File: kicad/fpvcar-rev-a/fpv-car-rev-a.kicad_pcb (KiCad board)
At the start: 2 copper layers, 58 parts, among them J1 CAMERA, J10 GPIO, J11 USB C, J12 GPIO, J13 GPIO, J14 RGB FL, J15 RGB FR, J16 RGB BL, J17 RGB BR, J2 Steering, J4 Battery, J5 Debug UART, J6 M1, J7 M2, J8 NRF24L01, J9 GPIO, Q1 Q_PMOS_GSD, SW1 SW_SPST, SW2 SW_SPST, U1 ESP32-S3-WROOM-1, U2 AMS1117-5.0, U3 XC6206-1.2V, U4 XC6206-2.8V, U5 DRV8833PWP, U6 WL2803K33-5/TR

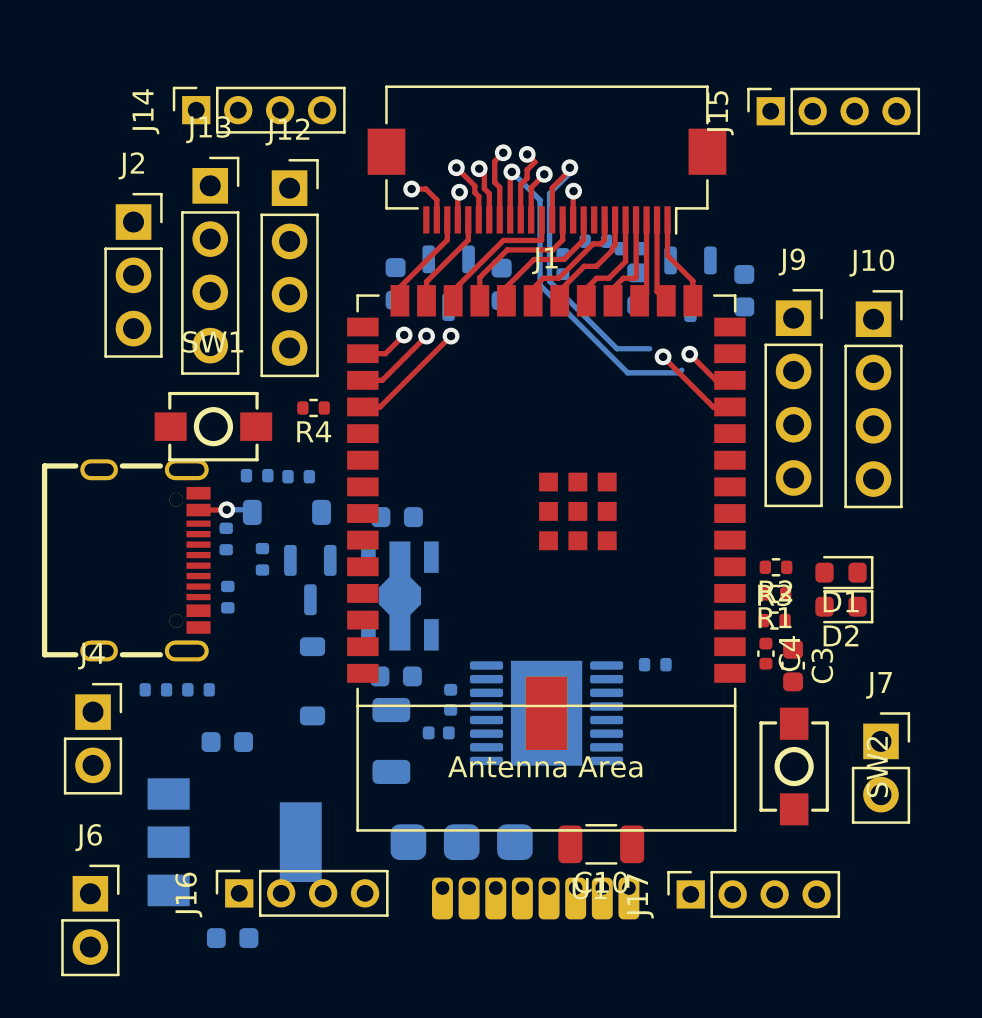
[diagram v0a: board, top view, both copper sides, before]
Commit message: PCB for rev. A done!
PCB name: S3Voyager :)
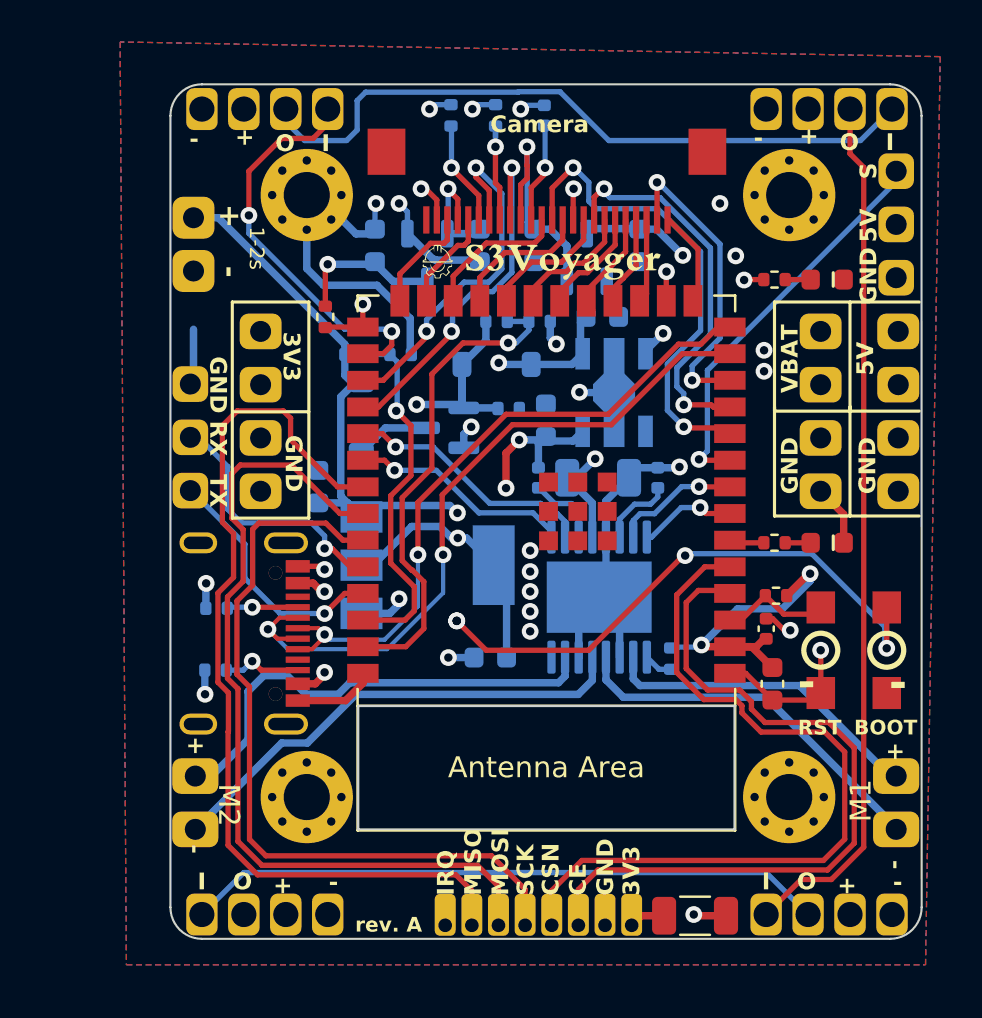
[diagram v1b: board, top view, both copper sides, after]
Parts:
- removed J10, J13: GPIO, Connector_PinSocket_2.54mm:PinSocket_1x04_P2.54mm_Vertical
- added H1: MountingHole_Pad, MountingHole:MountingHole_2.2mm_M2_Pad_Via, F.Cu at (164.0, 96.3)
- added H2: MountingHole_Pad, MountingHole:MountingHole_2.2mm_M2_Pad_Via, F.Cu at (141.0, 96.3)
- added H3: MountingHole_Pad, MountingHole:MountingHole_2.2mm_M2_Pad_Via, F.Cu at (141.0, 125.0)
- added H4: MountingHole_Pad, MountingHole:MountingHole_2.2mm_M2_Pad_Via, F.Cu at (164.0, 125.0)
- added J3: Bat Power, Custom3:conn_01x04, F.Cu at (165.5, 102.8)
- D1: renamed from D2; value BLUE -> RED
- D2: renamed from D1; value RED -> BLUE
- J12: value GPIO -> 3.3V Power; footprint Connector_PinSocket_2.54mm:PinSocket_1x04_P2.54mm_Vertical -> Custom3:conn_01x04
- J14, J15, J16, J17: footprint Connector_PinSocket_2.00mm:PinSocket_1x04_P2.00mm_Vertical -> Custom3:RGB_4_Pin_2mm_Female
- J9: value GPIO -> 5V Power; footprint Connector_PinSocket_2.54mm:PinSocket_1x04_P2.54mm_Vertical -> Custom3:conn_01x04
- moved J2 36.4 mm to (169.1, 95.2)
- moved SW1 33.8 mm to (168.7, 118.0), turned to -90 degrees
- moved J4 24.1 mm to (135.6, 97.4)
- moved J5 19.7 mm to (135.4, 110.4), turned to 0 degrees
- moved R12 18.7 mm to (145.5, 103.9)
- moved R11 18.6 mm to (143.3, 103.9)
- moved C1 18.2 mm to (149.8, 118.3)
- moved U2 16.1 mm to (146.8, 113.9)
- moved C9 16.0 mm to (154.9, 109.8), turned to 0 degrees
- moved C11 14.5 mm to (157.7, 109.8), turned to -90 degrees
- moved C15 14.1 mm to (152.4, 107.0), turned to 90 degrees
- moved U6 14.1 mm to (155.7, 105.7)
- moved D2 14.0 mm to (165.8, 100.3)
- moved R10 13.8 mm to (150.6, 106.5), turned to 0 degrees
- moved R2 13.7 mm to (163.3, 100.3), turned to 0 degrees
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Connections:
- net NRF_IRQ renamed /NRF_IRQ
- D1 pad 2: Net-(D2-A) -> Net-(D1-A)
- D2 pad 2: Net-(D1-A) -> Net-(D2-A)
- J12 pad 1: GPIO00 -> +3.3V
- J12 pad 2: GPIO00 -> +3.3V
- J12 pad 3: +3.3V -> GND
- J16 pad 1: /RGB_FR_BL -> /RGB_BL_BR
- J16 pad 2: /RGB_BL_BR -> unconnected-(J16-Pin_2-Pad2)
- J17 pad 1: /RGB_BL_BR -> /RGB_FR_BL
- J17 pad 2: unconnected-(J17-Pin_2-Pad2) -> /RGB_BL_BR
- J6 pad 1: MOTOR_A_OUT1 -> MOTOR_B_OUT1
- J6 pad 2: MOTOR_A_OUT2 -> MOTOR_B_OUT2
- J7 pad 1: MOTOR_B_OUT1 -> MOTOR_A_OUT1
- J7 pad 2: MOTOR_B_OUT2 -> MOTOR_A_OUT2
- J9 pad 1: GPIO00 -> +5V
- J9 pad 2: GPIO00 -> +5V
- J9 pad 3: +5V -> GND
- U1 pad 10: unconnected-(U1-GPIO17/U1TXD/ADC2_CH6-Pad10) -> XCLK
- U1 pad 11: unconnected-(U1-GPIO18/U1RXD/ADC2_CH7/CLK_OUT3-Pad11) -> PCLK
- U1 pad 12: unconnected-(U1-GPIO8/TOUCH8/ADC1_CH7/SUBSPICS1-Pad12) -> DATA1
- U1 pad 16: DATA1 -> LED_BLUE
- U1 pad 28: unconnected-(U1-SPIIO6/GPIO35/FSPID/SUBSPID-Pad28) -> RGB_LED
- U1 pad 29: unconnected-(U1-SPIIO7/GPIO36/FSPICLK/SUBSPICLK-Pad29) -> VSYNC
- U1 pad 30: unconnected-(U1-SPIDQS/GPIO37/FSPIQ/SUBSPIQ-Pad30) -> HREF
- U1 pad 31: unconnected-(U1-GPIO38/FSPIWP/SUBSPIWP-Pad31) -> MOTOR_B_IN2
- U1 pad 32: unconnected-(U1-MTCK/GPIO39/CLK_OUT3/SUBSPICS1-Pad32) -> MOTOR_B_IN1
- U1 pad 33: unconnected-(U1-MTDO/GPIO40/CLK_OUT2-Pad33) -> NRF_MISO
- U1 pad 34: unconnected-(U1-MTDI/GPIO41/CLK_OUT1-Pad34) -> NRF_MOSI
- U1 pad 35: unconnected-(U1-MTMS/GPIO42-Pad35) -> NRF_SCK
- U1 pad 38: unconnected-(U1-GPIO2/TOUCH2/ADC1_CH1-Pad38) -> BATT_VOLTAGE
- U1 pad 39: unconnected-(U1-GPIO1/TOUCH1/ADC1_CH0-Pad39) -> USB_SENSE
- U1 pad 4: unconnected-(U1-GPIO4/TOUCH4/ADC1_CH3-Pad4) -> NRF_CE
- U1 pad 5: unconnected-(U1-GPIO5/TOUCH5/ADC1_CH4-Pad5) -> NRF_CSN
- U1 pad 6: unconnected-(U1-GPIO6/TOUCH6/ADC1_CH5-Pad6) -> LED_RED
- U1 pad 7: unconnected-(U1-GPIO7/TOUCH7/ADC1_CH6-Pad7) -> MOTOR_A_IN1
- U1 pad 8: unconnected-(U1-GPIO15/U0RTS/ADC2_CH4/XTAL_32K_P-Pad8) -> MOTOR_A_IN2
- U1 pad 9: unconnected-(U1-GPIO16/U0CTS/ADC2_CH5/XTAL_32K_N-Pad9) -> STEER
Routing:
- net GND: track 3.75 -> 204.9 mm, vias 2 -> 26
- net +5V: track 0.00 -> 148.6 mm, vias 0 -> 1
- net +3.3V: track 2.43 -> 136.2 mm, vias 1 -> 8
- net VBAT: track 0.00 -> 54.7 mm, vias 0 -> 2
- net ~{BOOT}: track 0.00 -> 50.1 mm, vias 0 -> 5
- net NRF_MISO: track 0.00 -> 44.0 mm
- net /RGB_FR_BL: track 0.00 -> 41.5 mm
- net NRF_MOSI: track 0.00 -> 41.0 mm
- net NRF_CSN: track 0.00 -> 37.4 mm
- net NRF_SCK: track 0.00 -> 36.9 mm
- net NRF_CE: track 0.00 -> 35.6 mm
- net USB-: track 0.00 -> 34.3 mm, vias 0 -> 2
- net /RGB_FL_FR: track 0.00 -> 33.8 mm
- net USB+: track 0.00 -> 31.5 mm, vias 0 -> 2
- net /RGB_BL_BR: track 0.00 -> 30.6 mm
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- added copper zone on In2.Cu, net +3.3V
- added copper zone on B.Cu, net GND
- added copper zone on F.Cu, net GND
- added copper zone on In1.Cu, net GND
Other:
- board outline added: 35.8 x 40.7 mm
- copper layers 2 -> 4
- board text added: "+"
- board text added: "-"
- board text added: "1-2s"
- board text added: "3V3"
- board text added: "5V"
- board text added: "BOOT"
- board text added: "CE"
- board text added: "CSN"
- board text added: "Camera"
- board text added: "GND"
- board text added: "I"
- board text added: "IRQ"
- board text added: "M1"
- board text added: "M2"
- board text added: "MISO"
- board text added: "MOSI"
- board text added: "O"
- board text added: "RST"
- board text added: "RX"
- board text added: "S"
- board text added: "SCK"
- board text added: "TX"
- board text added: "VBAT"
- board text added: "Why did the RC car stop talking to its remote? Because it felt like it was being controlled too much"
- board text added: "rev. A"
